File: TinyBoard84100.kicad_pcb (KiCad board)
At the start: 2 copper layers, 13 parts, among them P2 CONN_01X07, P3 CONN_01X07, P4 CONN_02X03, SW1 SW_PUSH, U1 78L05, U2 ATTINY841

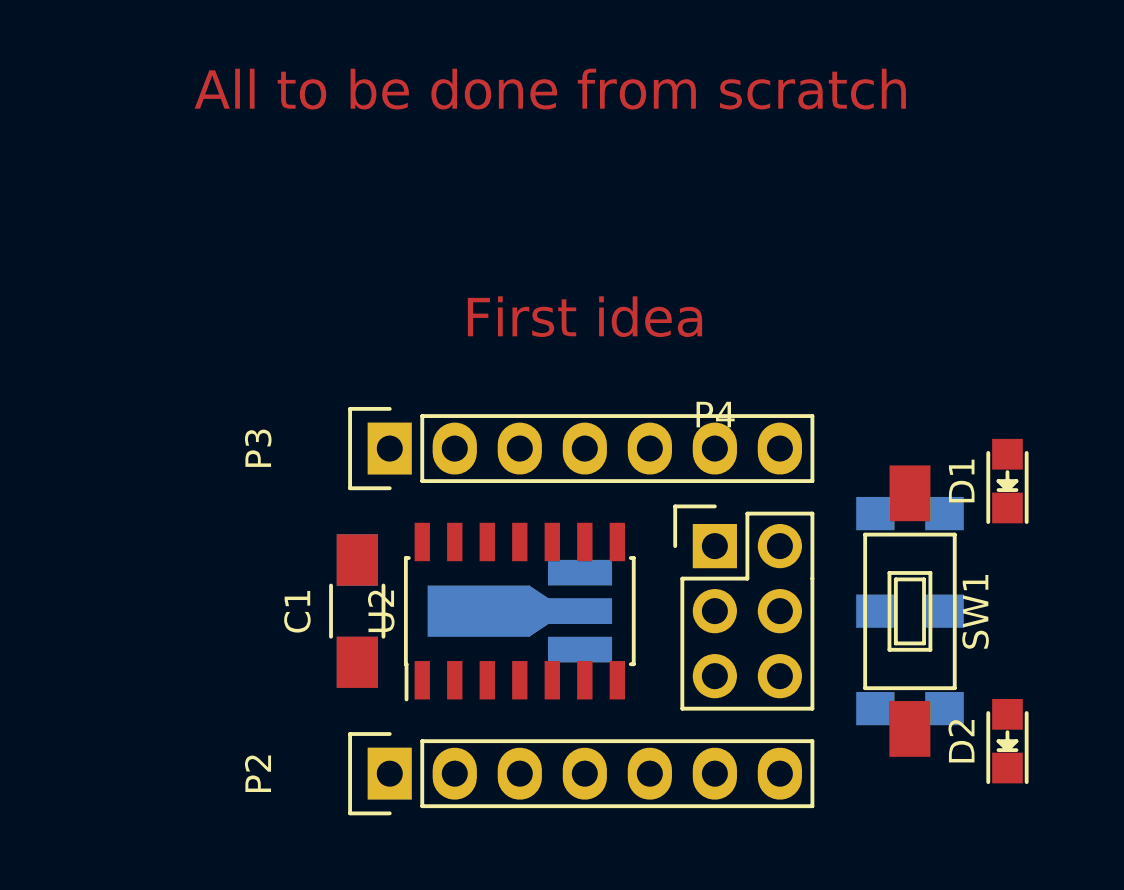
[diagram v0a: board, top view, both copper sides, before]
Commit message: almost finished layout
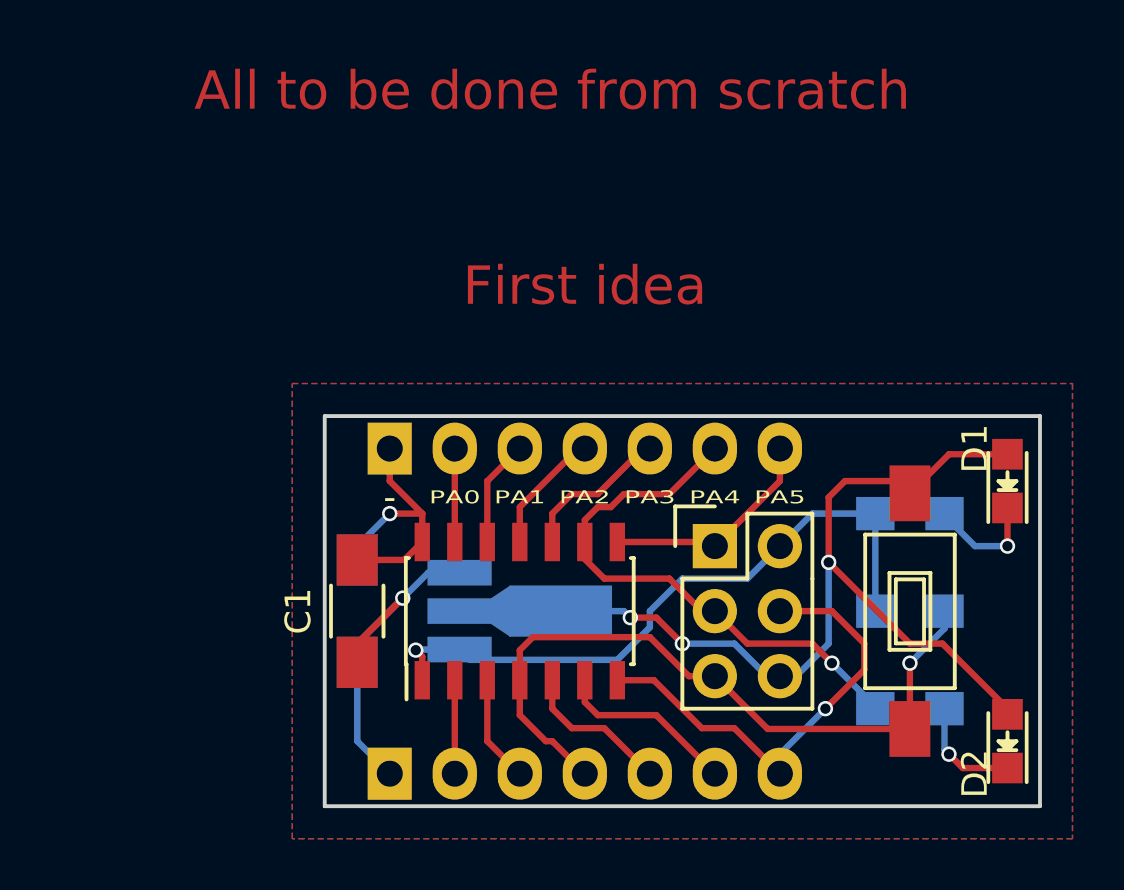
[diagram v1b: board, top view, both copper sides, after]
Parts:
- P2, P3: moved to B.Cu
- turned P2 to 270 degrees
- turned P3 to 270 degrees
- turned U1 to 90 degrees
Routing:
- net GND: track 0.00 -> 46.0 mm, vias 0 -> 4
- net /PB3: track 0.00 -> 28.1 mm, vias 0 -> 1
- net +5V: track 0.00 -> 26.0 mm, vias 0 -> 1
- net /PA4: track 0.00 -> 21.6 mm, vias 0 -> 1
- net /PA6: track 0.00 -> 18.1 mm, vias 0 -> 1
- net +BATT: track 0.00 -> 16.5 mm, vias 0 -> 1
- net /PA5: track 0.00 -> 8.74 mm
- net /PA7: track 0.00 -> 7.09 mm
- net /PA3: track 0.00 -> 5.97 mm
- net /PB2: track 0.00 -> 5.97 mm
- net /PA2: track 0.00 -> 4.85 mm
- net Net-(D1-Pad1): track 0.00 -> 4.52 mm, vias 0 -> 1
- net Net-(D2-Pad1): track 0.00 -> 4.36 mm, vias 0 -> 1
- net /PB1: track 0.00 -> 4.18 mm
- net /PA1: track 0.00 -> 4.18 mm
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- added copper zone on F.Cu, net +5V
- added copper zone on B.Cu, net GND
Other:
- board outline added: 27.9 x 15.2 mm
- board text added: "-"
- board text added: "PA0"
- board text added: "PA1"
- board text added: "PA2"
- board text added: "PA3"
- board text added: "PA4"
- board text added: "PA5"
